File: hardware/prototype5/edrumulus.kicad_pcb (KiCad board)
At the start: 4 copper layers, 65 x 56.5 mm, 100 parts, among them J1 Trigger Connector, J2 Raspberry Pi GPIO pins, U1 ESP32-WROOM-32U, U2 AMS1117-3.3, U3 MCP1754S-3302xMB

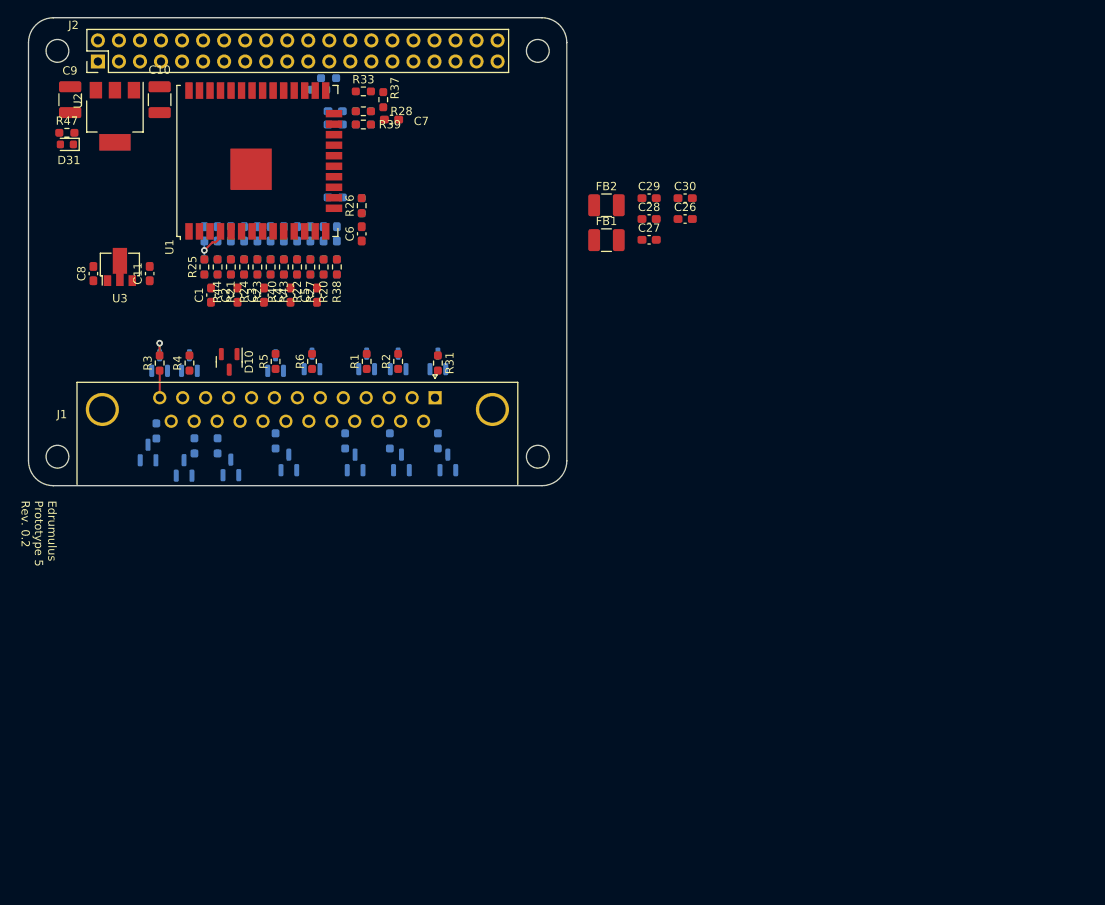
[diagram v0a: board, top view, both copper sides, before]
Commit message: delivery jstma for prototype 5 on 8/28/2022
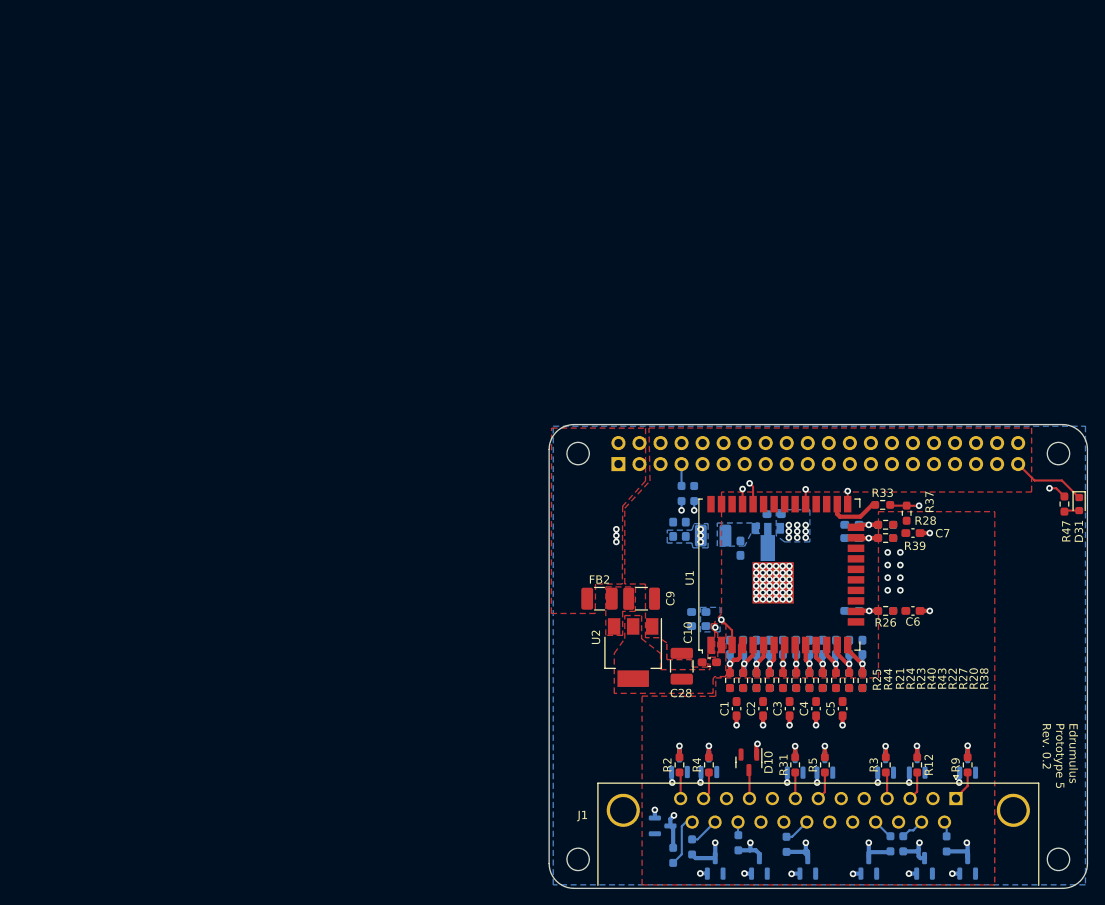
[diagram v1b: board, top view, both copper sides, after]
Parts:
- added MH1: MountingHole_2.7mm_M2.5, MountingHole:MountingHole_2.7mm_M2.5, F.Cu at (172.9, 125.7)
- added MH2: MountingHole_2.7mm_M2.5, MountingHole:MountingHole_2.7mm_M2.5, F.Cu at (230.9, 125.7)
- added MH3: MountingHole_2.7mm_M2.5, MountingHole:MountingHole_2.7mm_M2.5, F.Cu at (172.9, 174.7)
- added MH4: MountingHole_2.7mm_M2.5, MountingHole:MountingHole_2.7mm_M2.5, F.Cu at (230.9, 174.7)
- C11, C26, C27, C29, C30, C8, FB1, R1, R6, U3: moved to B.Cu
- J2: footprint Connector_PinHeader_2.54mm:PinHeader_2x20_P2.54mm_Vertical -> Connector_PinSocket_2.54mm:PinSocket_2x20_P2.54mm_Vertical; moved to B.Cu
- R12, R9: moved to F.Cu
- moved D31 129.7 mm to (233.4, 131.8), turned to -90 degrees
- moved R47 128.5 mm to (231.6, 131.8), turned to -90 degrees
- moved R9 105.9 mm to (220.0, 163.3)
- moved D9 105.9 mm to (220.0, 163.3)
- moved R3 100.2 mm to (210.1, 163.3)
- moved D3 100.2 mm to (210.1, 163.3)
- moved R8 96.8 mm to (210.6, 172.8)
- moved D7 96.6 mm to (214.8, 175.5)
- moved R7 95.7 mm to (212.2, 172.8)
- moved D8 95.6 mm to (208.0, 175.5)
- moved D12 95.3 mm to (220.0, 175.5)
- moved R29 94.5 mm to (217.4, 172.9)
- moved C10 93.0 mm to (185.4, 151.4)
- moved C9 91.6 mm to (180.6, 143.3), turned to 0 degrees
- moved U2 90.1 mm to (179.6, 149.8)
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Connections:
- C12 pad 1: GPIO36 -> GPIO14
- C20 pad 1: GPIO14 -> GPIO36
- D2 pad 3: GPIO14 -> GPIO36
- D3 pad 3: GPIO36 -> GPIO14
- J1 pad 0: (no net) -> unconnected-(J1-Pad0)
- R1 pad 1: SNARE-RING -> RIDE-TIP
- R10 pad 1: GPIO36 -> GPIO14
- R12 pad 2: TOM2-TIP -> SNARE-TIP
- R16 pad 1: GPIO14 -> GPIO36
- R2 pad 1: SNARE-TIP -> CRASH1-RING
- R2 pad 2: GPIO14 -> GPIO36
- R20 pad 2: GPIO36 -> GPIO14
- R25 pad 2: GPIO14 -> GPIO36
- R29 pad 2: TOM3-TIP -> TOM1-TIP
- R3 pad 1: CRASH1-RING -> SNARE-RING
- R3 pad 2: GPIO36 -> GPIO14
- R31 pad 2: KICK-TIP -> HI-HAT-RING
- R35 pad 1: TOM1-RING -> TOM3-TIP
- R36 pad 1: TOM1-TIP -> RIDE-BELL-TIP
- R5 pad 1: HI-HAT-RING -> HI-HAT-TIP
- R6 pad 1: HI-HAT-TIP -> RIDE-RING
- R7 pad 1: RIDE-RING -> TOM1-RING
- R8 pad 1: RIDE-TIP -> TOM2-TIP
- R9 pad 1: RIDE-BELL-TIP -> KICK-TIP
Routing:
- net HI-HAT-CONTROL-TIP: track 0.00 -> 94.4 mm, vias 0 -> 1
- net GPIO15: track 0.00 -> 53.4 mm, vias 0 -> 2
- net GPIO13: track 0.00 -> 42.3 mm, vias 0 -> 2
- net GPIO2: track 0.00 -> 41.9 mm, vias 0 -> 2
- net PI-GPIO9: track 0.00 -> 39.2 mm, vias 0 -> 2
- net GPIO32: track 0.00 -> 37.3 mm, vias 0 -> 2
- net GPIO35: track 0.00 -> 35.9 mm, vias 0 -> 2
- net GPIO27: track 0.00 -> 33.9 mm, vias 0 -> 2
- net Net-(R47-Pad1): track 0.00 -> 33.9 mm, vias 0 -> 2
- net GPIO25: track 0.00 -> 33.6 mm, vias 0 -> 2
- net GPIO39: track 0.00 -> 32.7 mm, vias 0 -> 2
- net PI-GPIO4: track 0.00 -> 28.5 mm, vias 0 -> 1
- net GPIO12: track 0.00 -> 21.8 mm, vias 0 -> 2
- net GPIO34: track 0.00 -> 20.9 mm, vias 0 -> 2
- net GPIO14: track 0.00 -> 20.8 mm, vias 0 -> 2
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- added copper zone on B.Cu, net 3V3
- added copper zone on F.Cu, net 3V3
- added copper zone on In2.Cu, net 3V3
- added copper zone on B.Cu, net ESP32-3V3
- added copper zone on F.Cu, net ESP32-3V3
- added copper zone on B.Cu, net GND
- added copper zone on F.Cu, net GND
- added copper zone on In1.Cu, net GND
- added copper zone on B.Cu, net Net-(C8-Pad1)
- added copper zone on F.Cu, net Net-(C9-Pad1)
- added copper zone on B.Cu, net RASPI-VIN
- added copper zone on F.Cu, net RASPI-VIN
- added copper zone on In1.Cu, net RASPI-VIN
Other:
- board size 65 x 56.5 mm -> 65 x 56 mm
- board text added: "J2 comes with pi hat mounting template. All parts placed with reference to pin1 of J2."
- board text added: "TODO: Vias under esp32 gnd pad must be untented. Vias in the pad of FB1 must be untented too. Meanwhile the rest of the vias must be tented. pin 15 is not connected to ground. I don't think it needs to be, but if there is a problem it might be good to be able to ground that pin. I guess a wire can be added to the ground side of C6. Maybe beef up the wires from the db25 into the 100k resistor."
